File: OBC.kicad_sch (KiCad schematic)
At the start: 11 parts, among them J1 I2C, J6 SWD, J7 RMF, J8 GPIO, SW3 SW_Push, SW5 RST, U1 E73-2G4M08S1C, Y1 32.768

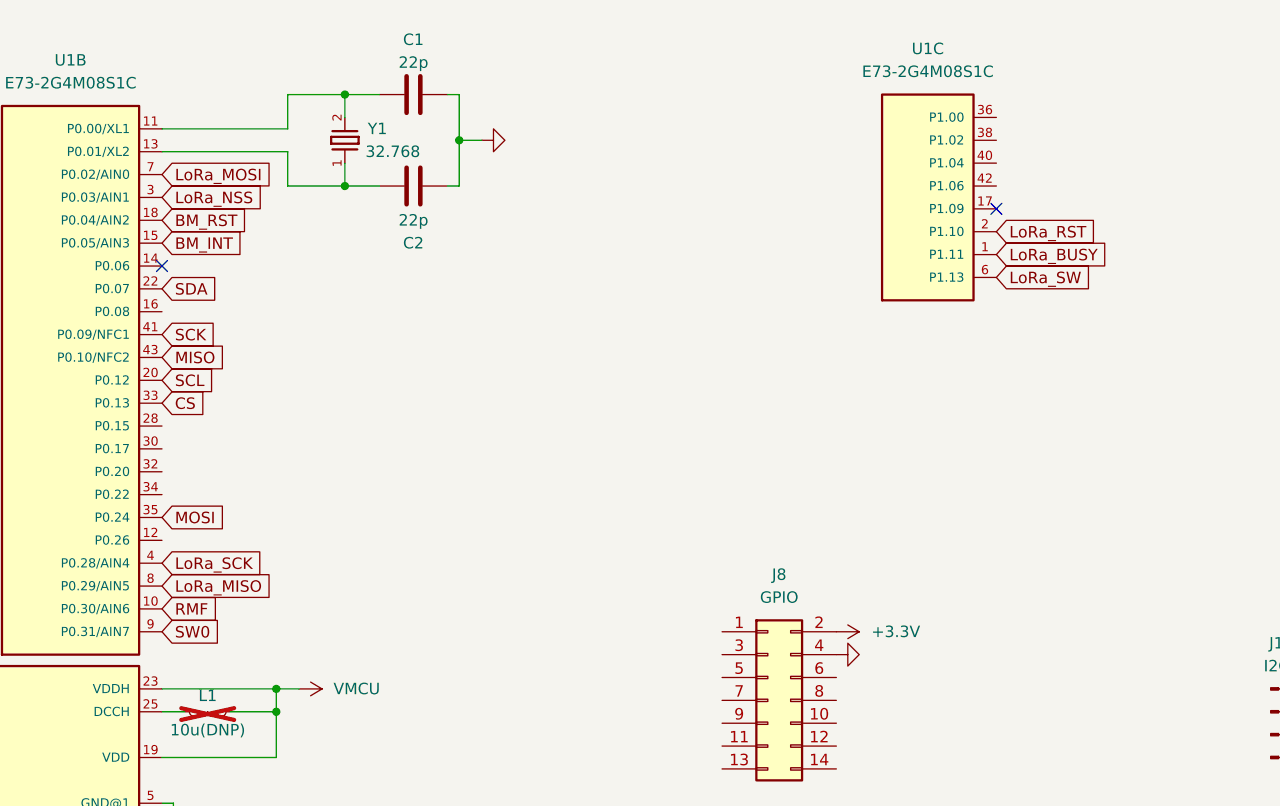
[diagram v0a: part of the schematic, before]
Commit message: Continued layout and routing
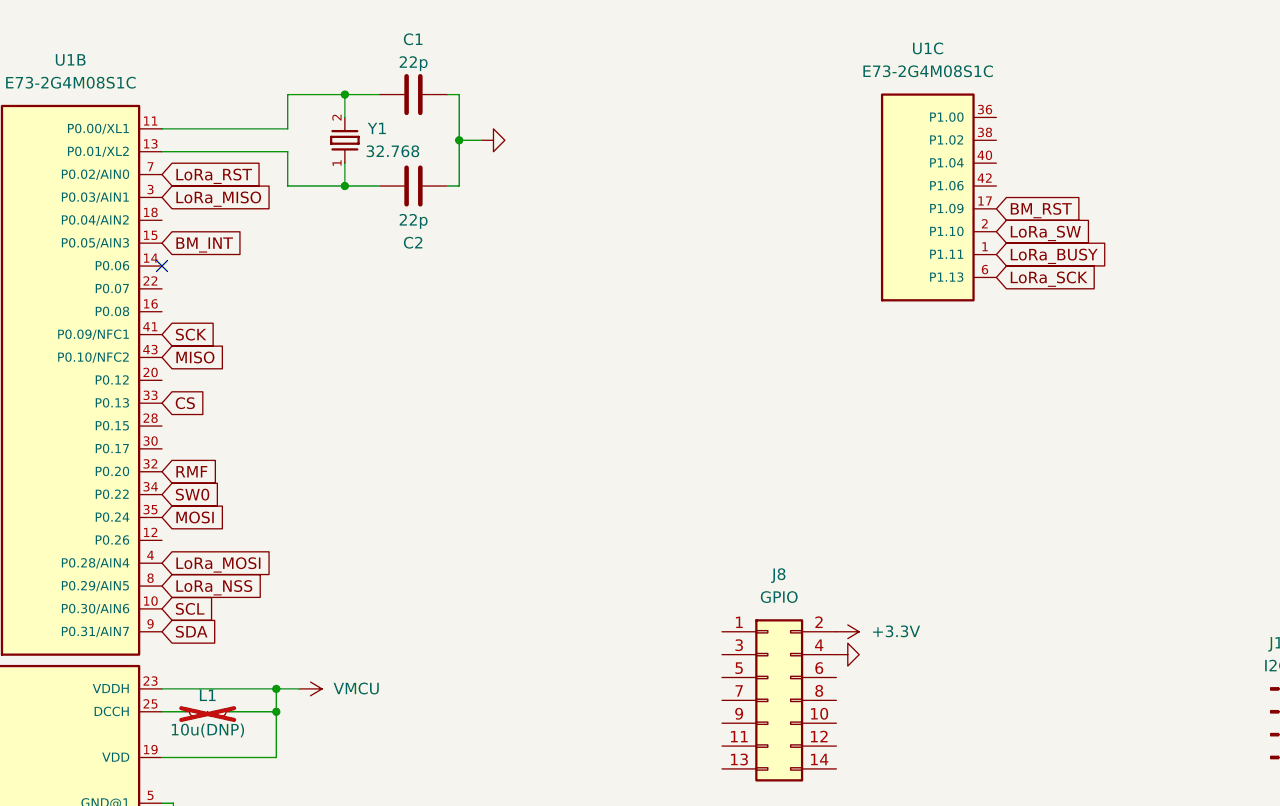
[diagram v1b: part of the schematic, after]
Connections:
- net BM_RST: now also U1.17 (P1.09); no longer U1.18 (P0.04/AIN2)
- net LoRa_MISO: now also U1.3 (P0.03/AIN1); no longer U1.8 (P0.29/AIN5)
- net LoRa_MOSI: now also U1.4 (P0.28/AIN4); no longer U1.7 (P0.02/AIN0)
- net LoRa_NSS: now also U1.8 (P0.29/AIN5); no longer U1.3 (P0.03/AIN1)
- net LoRa_RST: now also U1.7 (P0.02/AIN0); no longer U1.2 (P1.10)
- net LoRa_SCK: now also U1.6 (P1.13); no longer U1.4 (P0.28/AIN4)
- net LoRa_SW: now also U1.2 (P1.10); no longer U1.6 (P1.13)
- net RMF: now also U1.32 (P0.20); no longer U1.10 (P0.30/AIN6)
- net SCL: now also U1.10 (P0.30/AIN6); no longer U1.20 (P0.12)
- net SDA: now also U1.9 (P0.31/AIN7); no longer U1.22 (P0.07)
- net SW0: now also U1.34 (P0.22); no longer U1.9 (P0.31/AIN7)
- no-connect marks 3 -> 2

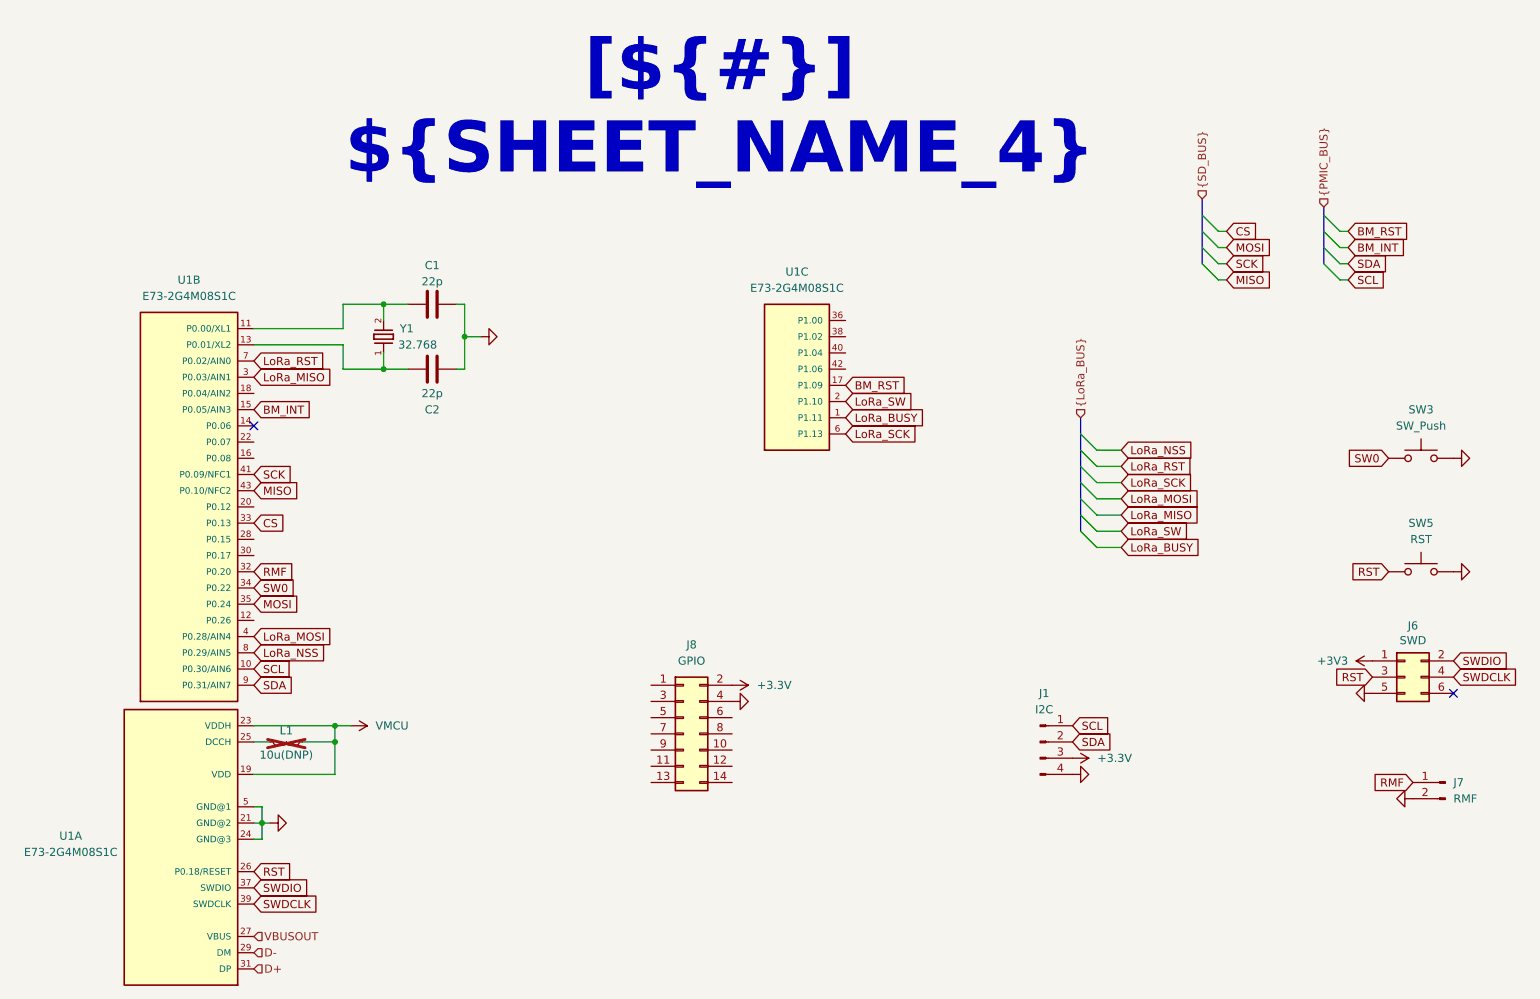
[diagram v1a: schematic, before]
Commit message: Finished PCB design
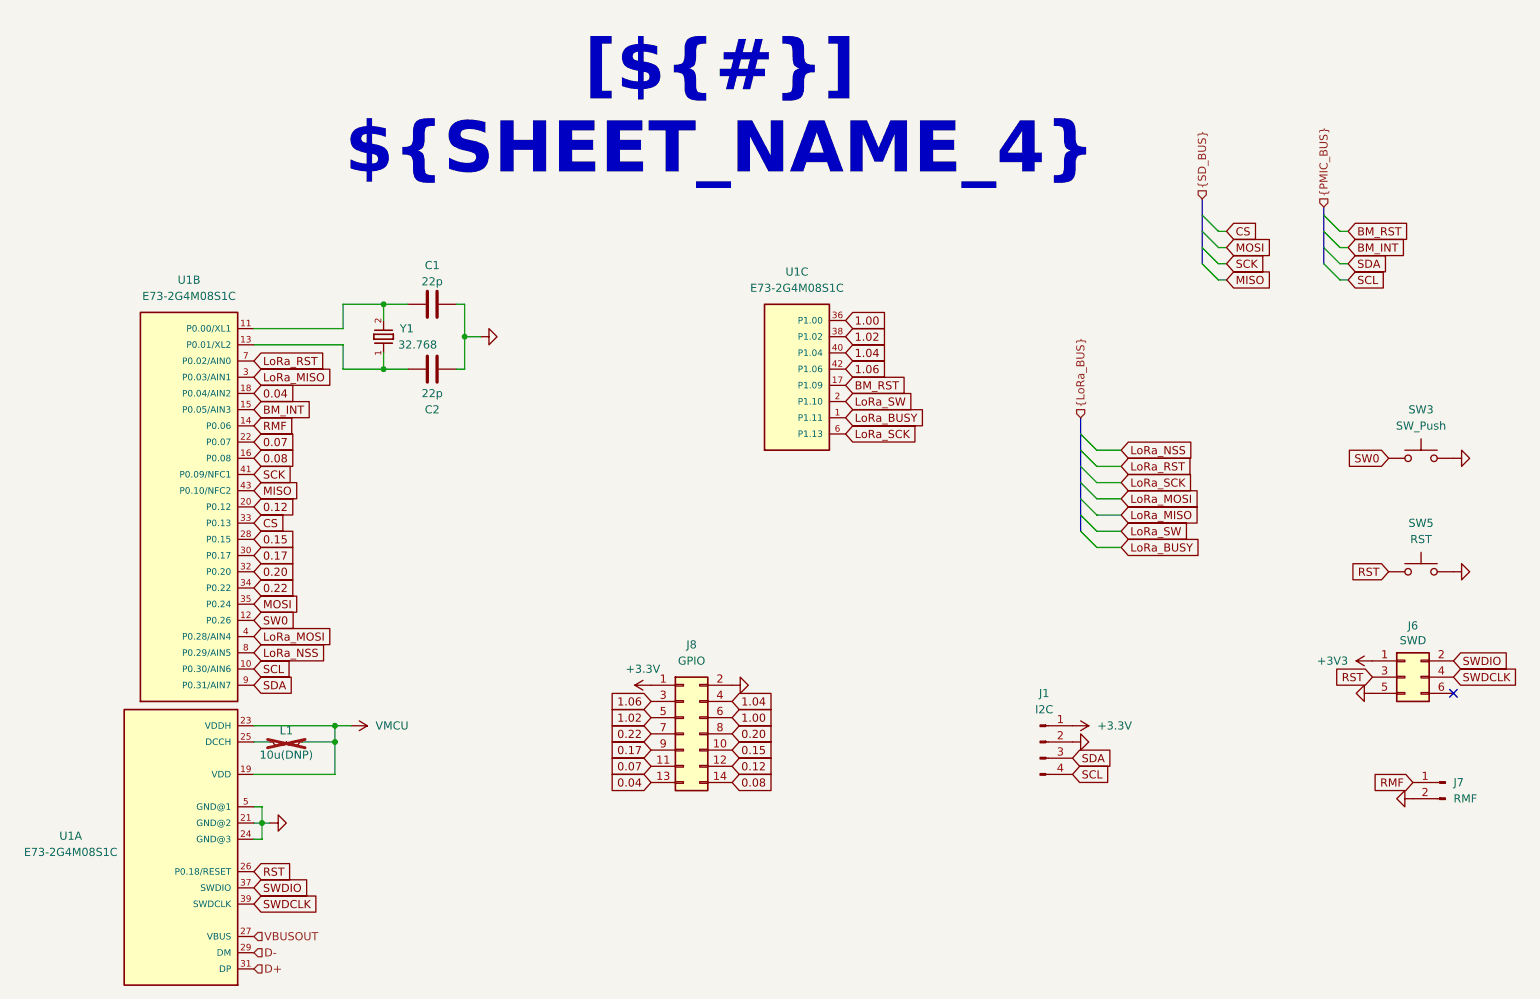
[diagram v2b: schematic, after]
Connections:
- net +3.3V: now also J1.1 (Pin_1), J8.1 (Pin_1); no longer J1.3 (Pin_3), J8.2 (Pin_2)
- net GND: now also J1.2 (Pin_2), J8.2 (Pin_2); no longer J1.4 (Pin_4), J8.4 (Pin_4)
- net RMF: now also U1.14 (P0.06); no longer U1.32 (P0.20)
- net SCL: now also J1.4 (Pin_4); no longer J1.1 (Pin_1)
- net SDA: now also J1.3 (Pin_3); no longer J1.2 (Pin_2)
- net SW0: now also U1.12 (P0.26); no longer U1.34 (P0.22)
- net 0.08: now reaches U1.16 (P0.08)
- net 0.08: now also J8.14 (Pin_14)
- net 0.04: now reaches U1.18 (P0.04/AIN2)
- net 0.04: now also J8.13 (Pin_13)
- net 0.12: now reaches U1.20 (P0.12)
- net 0.12: now also J8.12 (Pin_12)
- net 0.07: now reaches U1.22 (P0.07)
- net 0.07: now also J8.11 (Pin_11)
- net 0.15: now reaches U1.28 (P0.15)
- net 0.15: now also J8.10 (Pin_10)
- net 0.17: now reaches U1.30 (P0.17)
- net 0.17: now also J8.9 (Pin_9)
- net 1.06: now reaches J8.3 (Pin_3)
- net 1.06: now also U1.42 (P1.06)
- net 1.02: now reaches J8.5 (Pin_5)
- net 1.02: now also U1.38 (P1.02)
- net 1.00: now reaches J8.6 (Pin_6)
- net 1.00: now also U1.36 (P1.00)
- net 0.22: now reaches J8.7 (Pin_7)
- net 0.22: now also U1.34 (P0.22)
- net 0.20: now reaches J8.8 (Pin_8)
- net 0.20: now also U1.32 (P0.20)
- net 1.04: now reaches U1.40 (P1.04)
- net 1.04: now also J8.4 (Pin_4)
- no-connect marks 2 -> 1
